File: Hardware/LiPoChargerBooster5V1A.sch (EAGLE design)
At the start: 36 parts, among them J1 AMP FCI 10103594-0001LF, J2 PTH, J3 PTH, J4 JST, J7 PTH, U1 MCP73831, U2 PAM2401

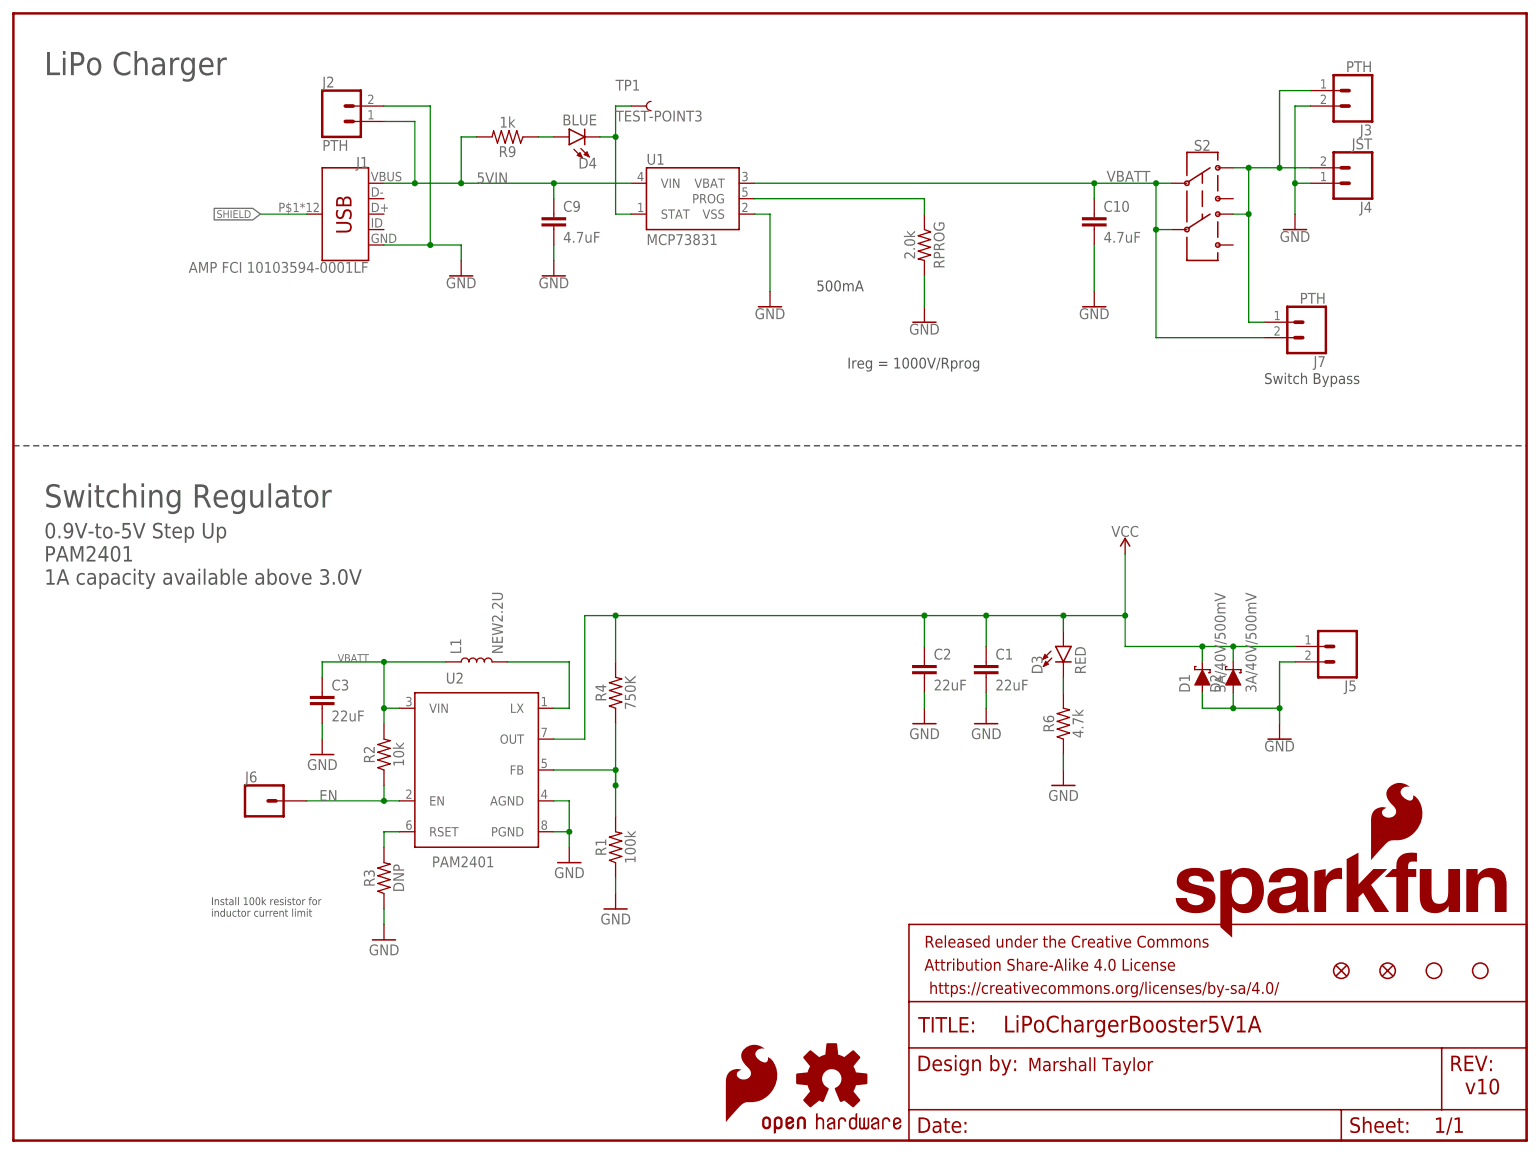
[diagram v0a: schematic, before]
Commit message: Post reivew changes
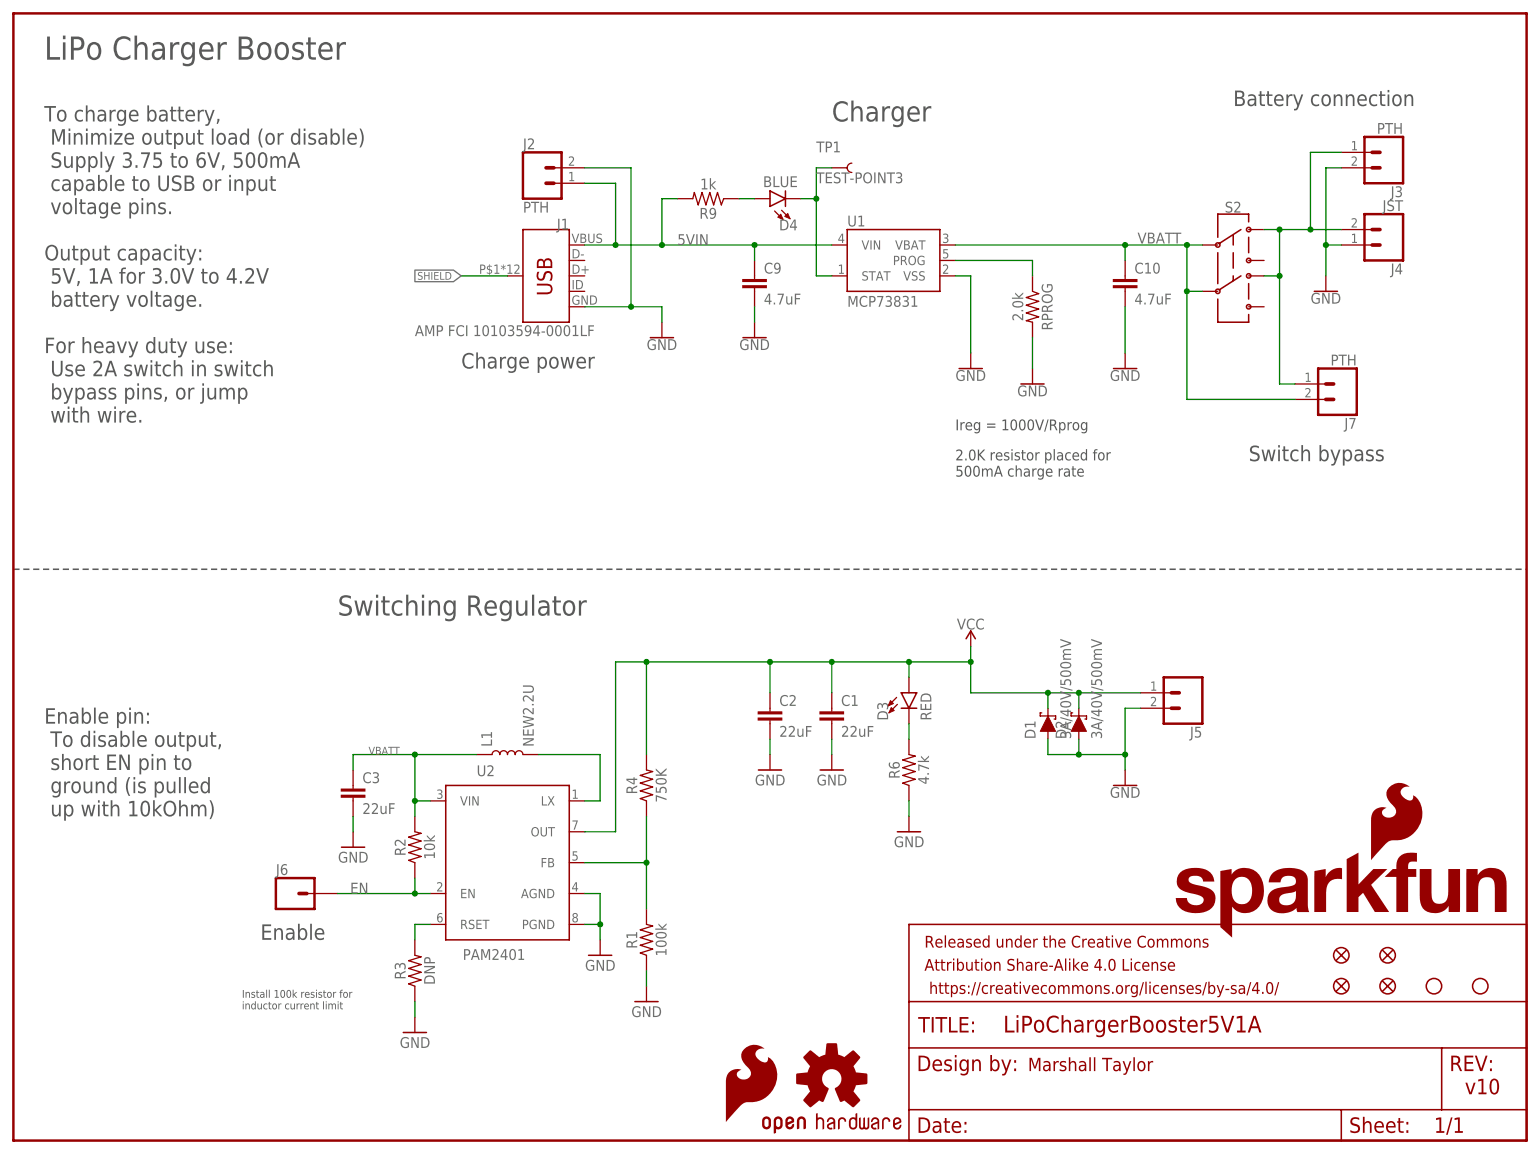
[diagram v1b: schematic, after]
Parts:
- added JP1, JP4: FIDUCIAL1X2, SparkFun-Aesthetics:FIDUCIAL1X2
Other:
- note added: "2.0K resistor placed for 500mA charge rate"
- note added: "Battery connection"
- note added: "Charge power"
- note added: "Charger"
- note added: "Enable"
- note added: "Enable pin: To disable output, short EN pin to ground (is pulled up with 10kOhm)"
- note added: "For heavy duty use: Use 2A switch in switch bypass pins, or jump with wire."
- note added: "LiPo Charger Booster"
- note added: "Output capacity: 5V, 1A for 3.0V to 4.2V battery voltage."
- note added: "Switch bypass"
- note added: "To charge battery, Minimize output load (or disable) Supply 3.75 to 6V, 500mA capable to USB or input voltage pins."
- note removed: "0.9V-to-5V Step Up PAM2401 1A capacity available above 3.0V"
- note removed: "500mA"
- note removed: "LiPo Charger"
- note removed: "Switch Bypass"
- moved on the sheet: C1, C10, C2, C3, C9, D1, D2, D3, D4, J1, J2, J3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
